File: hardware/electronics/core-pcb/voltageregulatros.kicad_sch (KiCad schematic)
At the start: 79 parts, among them IC5 BQ24133RGYR, IC6 LM5176PWPR, Q10 30V 71A, Q11 30V 71A, Q12 30V 71A, Q13 30V 71A, Q7 30V 71A, Q8 30V 71A, Q9 40V 70A, U1 LD1117S25TR_SOT223, U2 LD1117S33TR_SOT223, U3 LD1117S50TR_SOT223, U4 LD1117S50TR_SOT223

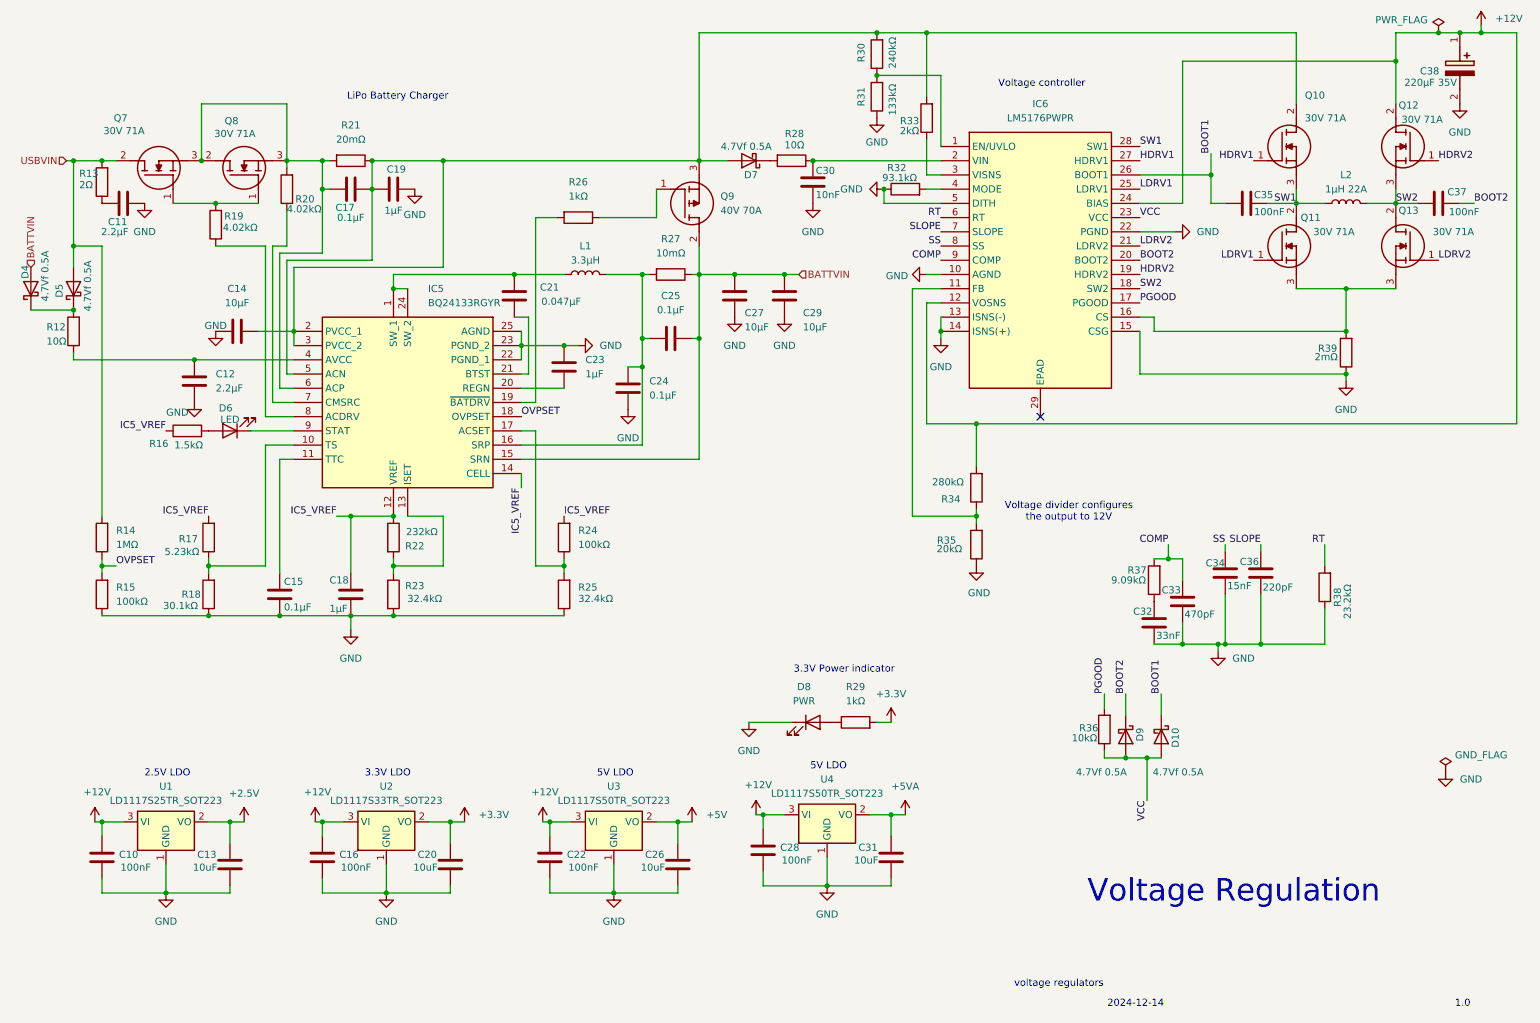
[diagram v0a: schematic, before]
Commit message: started work on pcbv2 work in progress
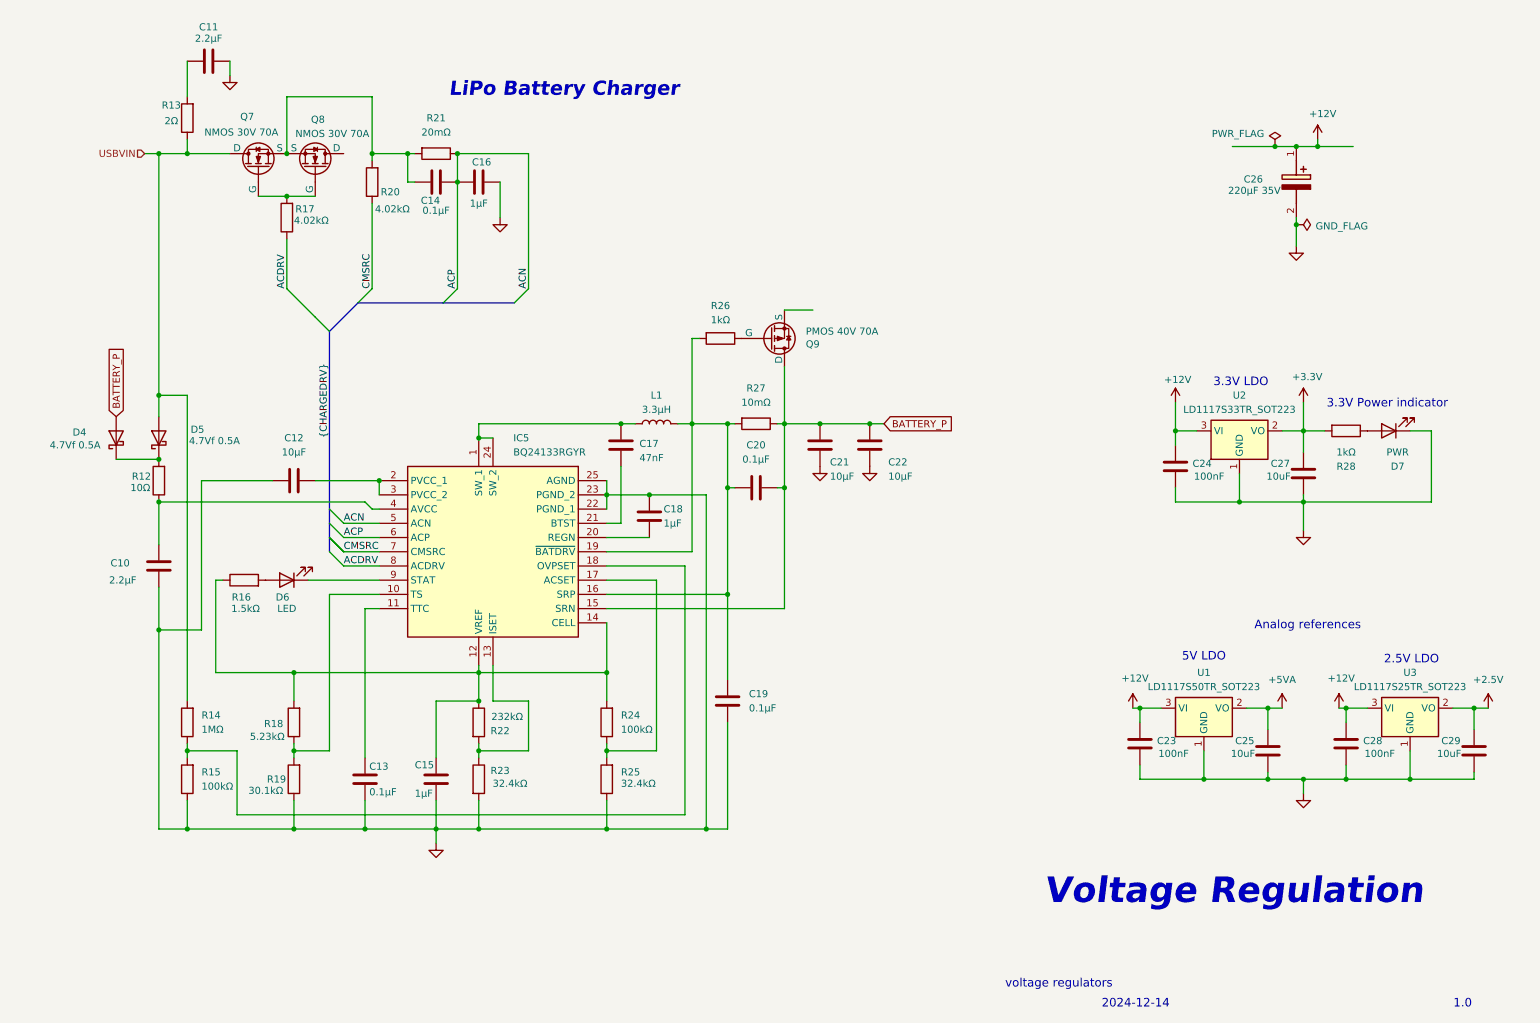
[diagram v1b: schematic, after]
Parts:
- removed C22, C35, C37: 100nF, Capacitor_SMD:C_0603_1608Metric, symbol Device:C
- removed C26: 10uF, Capacitor_SMD:C_0603_1608Metric, symbol Device:C
- removed C30: 10nF, Capacitor_SMD:C_0603_1608Metric, symbol Device:C
- removed C32: 33nF, Capacitor_SMD:C_0603_1608Metric, symbol Device:C
- removed C33: 470pF, Capacitor_SMD:C_0603_1608Metric, symbol Device:C
- removed C34: 15nF, Capacitor_SMD:C_0603_1608Metric, symbol Device:C
- removed C36: 220pF, Capacitor_SMD:C_0603_1608Metric, symbol Device:C
- removed D10, D7, D9: 4.7Vf 0.5A, kuben-footprints:DIOC1709X85N, symbol Device:D_Schottky
- removed IC6: LM5176PWPR, kuben-footprints:SOP65P640X120-29N, symbol LM5176PWPR:LM5176PWPR
- removed L2: 1µH 22A, kuben-footprints:INDPM6965X300N, symbol Device:L
- removed Q10, Q11, Q12, Q13, Q7, Q8: 30V 71A, kuben-footprints:IPD047N03LF2SATMA1, symbol IPD047N03LF2SATMA1:IPD047N03LF2SATMA1
- removed Q9: 40V 70A, kuben-footprints:IPD70P04P4L08ATMA2, symbol IPD70P04P4L08ATMA2:IPD70P04P4L08ATMA2
- removed R28: 10Ω, Resistor_SMD:R_0603_1608Metric, symbol Device:R
- removed R30: 240kΩ, Resistor_SMD:R_0603_1608Metric, symbol Device:R
- removed R31: 133kΩ, Resistor_SMD:R_0603_1608Metric, symbol Device:R
- removed R32: 93.1kΩ, Resistor_SMD:R_0603_1608Metric, symbol Device:R
- removed R33: 2kΩ, Resistor_SMD:R_0603_1608Metric, symbol Device:R
- removed R34: 280kΩ, Resistor_SMD:R_0603_1608Metric, symbol Device:R
- removed R35: 20kΩ, Resistor_SMD:R_0603_1608Metric, symbol Device:R
- removed R36: 10kΩ, Resistor_SMD:R_0603_1608Metric, symbol Device:R
- removed R37: 9.09kΩ, Resistor_SMD:R_0603_1608Metric, symbol Device:R
- removed R38: 23.2kΩ, Resistor_SMD:R_0603_1608Metric, symbol Device:R
- removed R39: 2mΩ, Resistor_SMD:R_0603_1608Metric, symbol Device:R
- removed U3: LD1117S50TR_SOT223, Package_TO_SOT_SMD:SOT-223-3_TabPin2, symbol Regulator_Linear:LD1117S50TR_SOT223
- added Q7, Q8: NMOS 30V 70A, footprints:IPD047N03LF2SATMA1, symbol Device:Q_NMOS
- added Q9: PMOS 40V 70A, footprints:IPD70P04P4L08ATMA2, symbol Device:Q_PMOS
- C17: renamed from C21; value 0.047µF -> 47nF
- renumbered C12 to C10, C14 to C12, C15 to C13, C17 to C14, C18 to C15, C19 to C16, C23 to C18, C24 to C19, C25 to C20, C27 to C21, C29 to C22, C28 to C23, C16 to C24, C31 to C25, C38 to C26, C20 to C27, C10 to C28, C13 to C29, D8 to D7, R19 to R17, R17 to R18, R18 to R19, R29 to R28, U4 to U1, U1 to U3
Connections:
- net GND: now also C12.1; no longer C12.2
- net USBVIN: now also R13.1, Q7.1 (D); no longer R13.2
- net at C14.1, R20.2, R21.2: now also Q7.3 (S), Q8.3 (S); no longer IC5.6 (ACP)
- net ACN: now reaches C14.2, C16.1, IC5.5 (ACN), R21.1
- net ACN: now also IC5.6 (ACP); no longer C12.1, IC5.2 (PVCC_1), IC5.3 (PVCC_2)
- net at R17.2: now also Q7.2 (G), Q8.2 (G)
- net at C19.2, C20.1, IC5.16 (SRP)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: now also IC5.19 (~{BATDRV}), R26.2
- net ACDRV: now reaches IC5.8 (ACDRV), R17.1
- net CMSRC: now reaches IC5.7 (CMSRC), R20.1
- net at C11.1: now also R13.2; no longer R13.1
- net at R26.1: now also Q9.1 (G)
- net BATTVIN renamed BATTERY_P
- net BATTERY_P: now also Q9.2 (D)
- net IC5_VREF: no longer names the net of C15.1, IC5.12 (VREF), IC5.14 (CELL), R16.1, R18.2, R22.1, R24.2
- net OVPSET: no longer names the net of IC5.18 (OVPSET), R14.1, R15.2
- new net: C12.2, IC5.2 (PVCC_1), IC5.3 (PVCC_2)
- no-connect marks 1 -> 0
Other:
- note added: "Analog references"
- note removed: "Voltage controller"
- note removed: "Voltage divider configures the output to 12V"
- moved on the sheet: C10, C11, C12, C13, C14, C15, C16, C17, C18, C19, C20, C21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
